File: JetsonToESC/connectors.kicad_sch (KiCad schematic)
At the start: 7 parts, among them J1 Conn_01x12, J2 Conn_01x03, J3 Conn_01x02

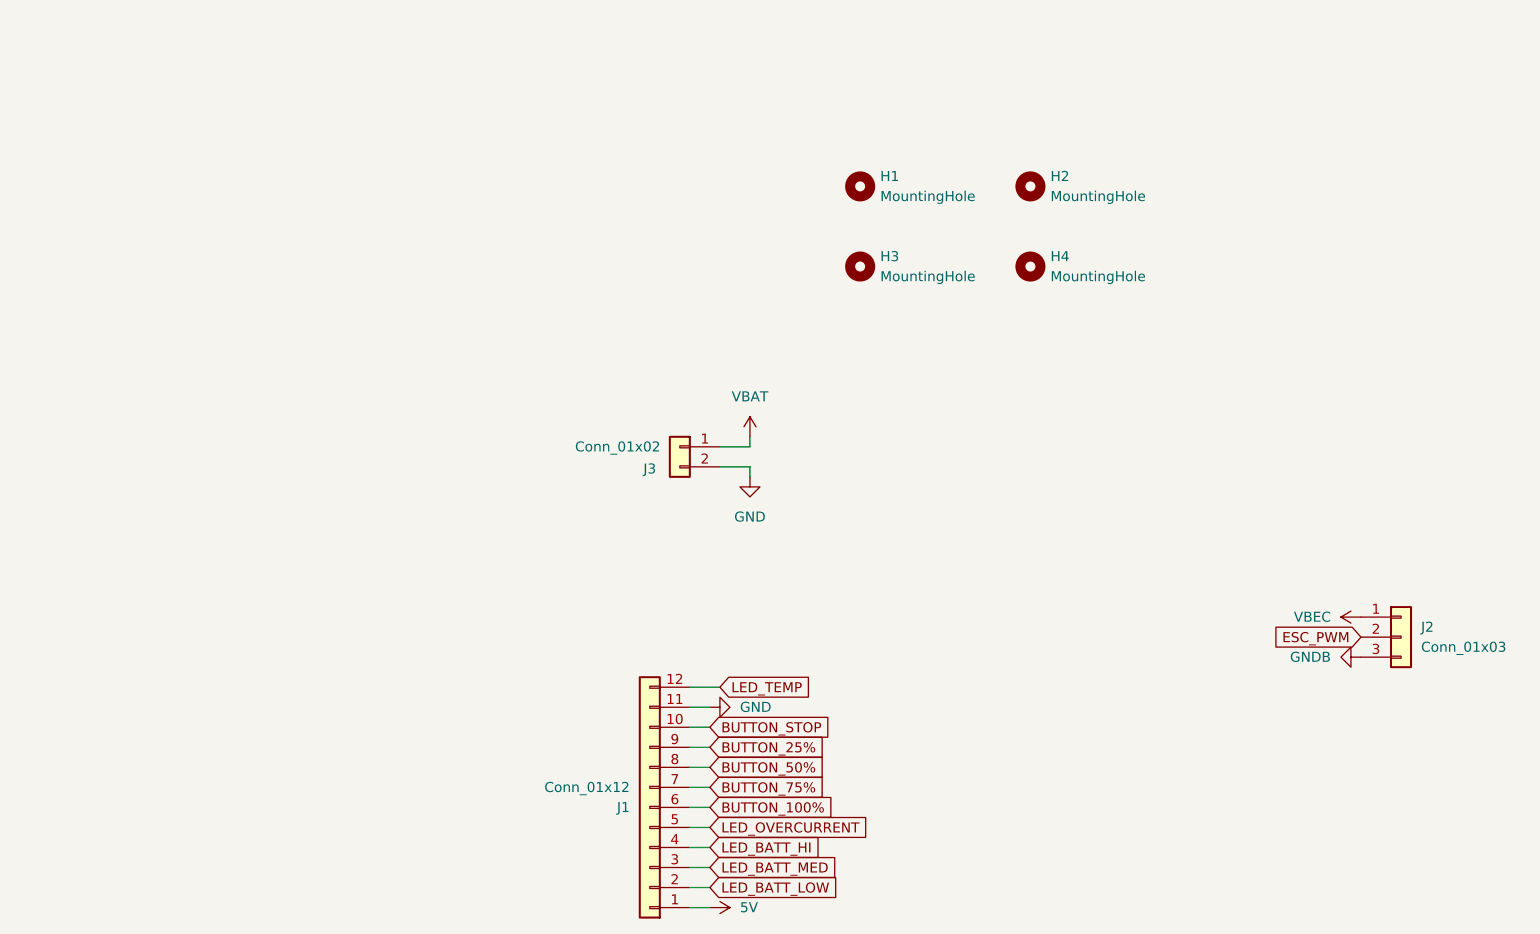
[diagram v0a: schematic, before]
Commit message: Start On this Branch
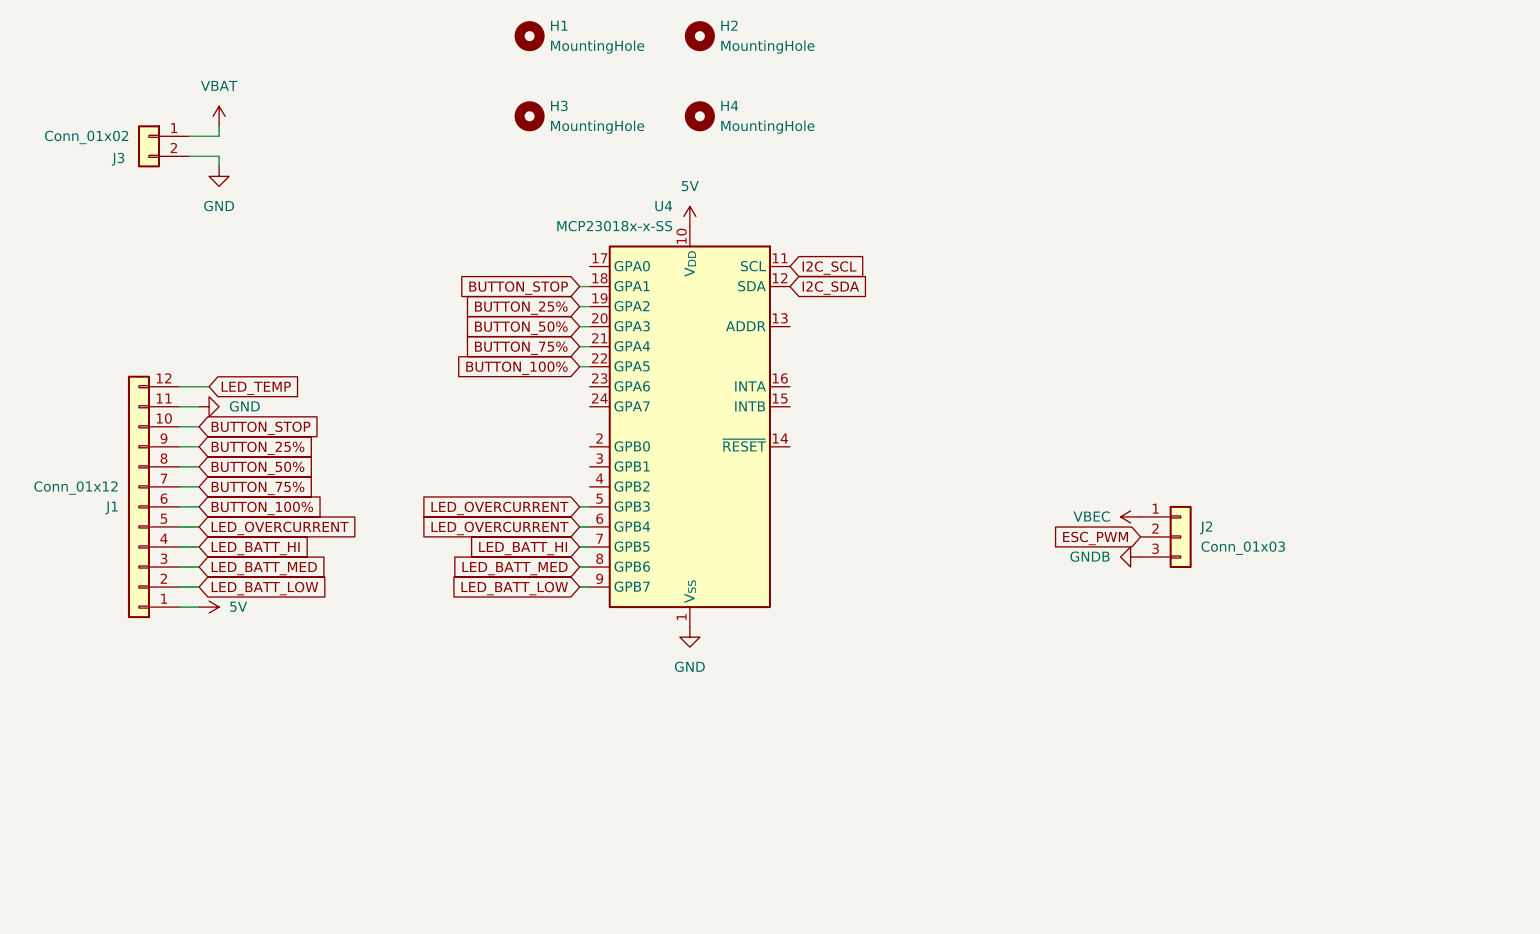
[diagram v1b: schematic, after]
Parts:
- added U4: MCP23018x-x-SS, Package_SO:SSOP-24_5.3x8.2mm_P0.65mm, symbol Interface_Expansion:MCP23018x-x-SS
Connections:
- net 5V: now also U4.10 (V_{DD})
- net BUTTON_100%: now also U4.22 (GPA5)
- net BUTTON_25%: now also U4.19 (GPA2)
- net BUTTON_50%: now also U4.20 (GPA3)
- net BUTTON_75%: now also U4.21 (GPA4)
- net BUTTON_STOP: now also U4.18 (GPA1)
- net GND: now also U4.1 (V_{SS})
- net LED_BATT_HI: now also U4.7 (GPB5)
- net LED_BATT_LOW: now also U4.9 (GPB7)
- net LED_BATT_MED: now also U4.8 (GPB6)
- net LED_OVERCURRENT: now also U4.5 (GPB3), U4.6 (GPB4)
- new net I2C_SCL: U4.11 (SCL)
- new net I2C_SDA: U4.12 (SDA)
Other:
- moved on the sheet: H1, H2, H3, H4, J1, J2, J3

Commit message: Work on current sense and io expansion branch
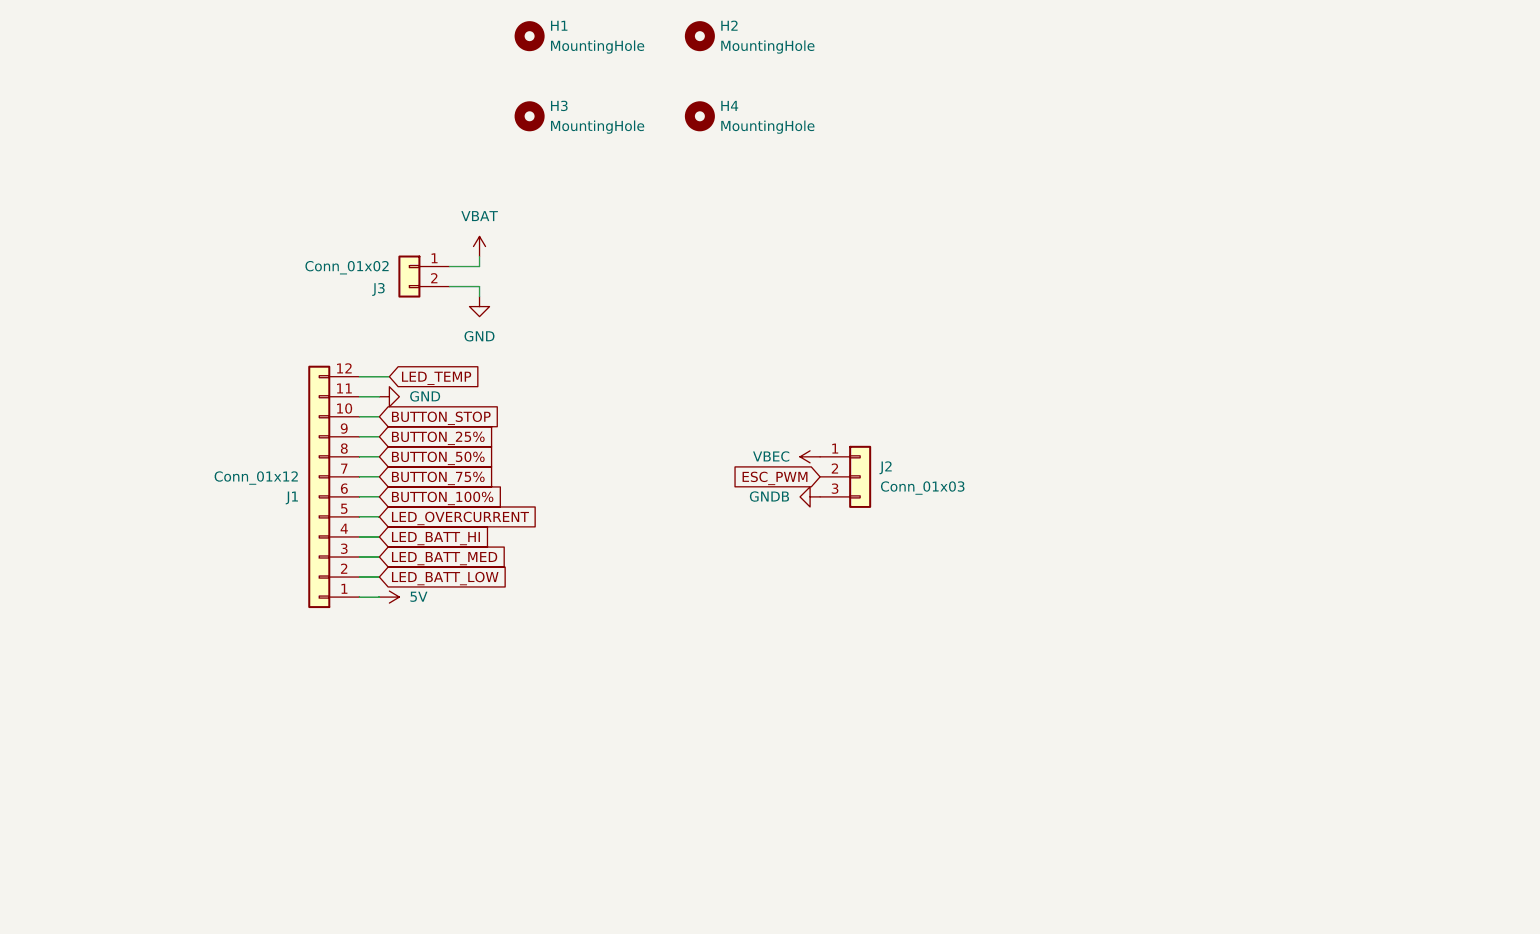
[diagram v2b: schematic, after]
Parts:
- removed U4: MCP23018x-x-SS, Package_SO:SSOP-24_5.3x8.2mm_P0.65mm, symbol Interface_Expansion:MCP23018x-x-SS
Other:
- moved on the sheet: J1, J2, J3
